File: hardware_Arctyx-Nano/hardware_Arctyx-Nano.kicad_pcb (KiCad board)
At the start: 4 copper layers, 21 x 51 mm, 74 parts, among them J1 USB_C_Receptacle_USB2.0_16P, J2 Conn_01x20_Pin, J3 Conn_01x20_Pin, SW1 SW_Push, U1 ICE40UP5K-SG48ITR, U2 RP2350A-QFN60, U3 W25Q128JVP, U4 RT8075ZQW, U5 TJ-S1608SW6TDSLCCYRGB-A5, Y1 Crystal_GND24

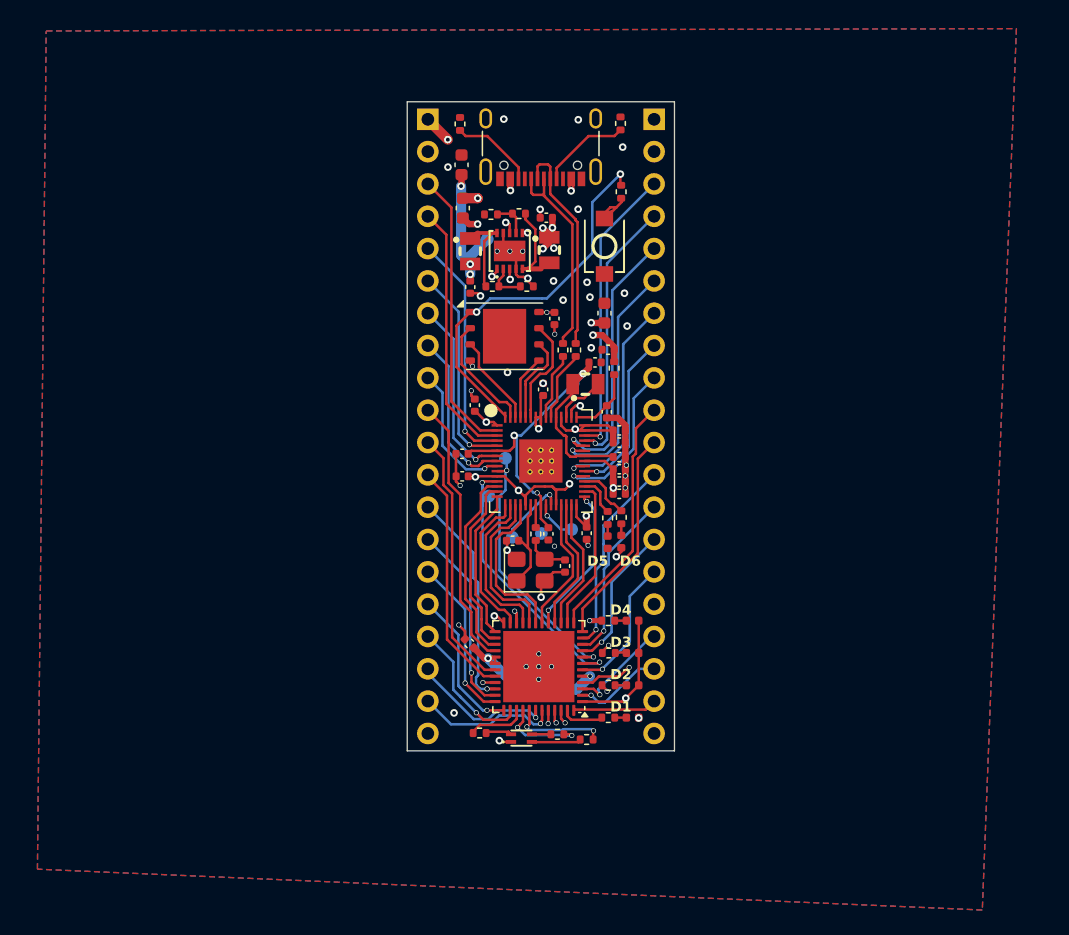
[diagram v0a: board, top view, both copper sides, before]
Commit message: production files generation and branding
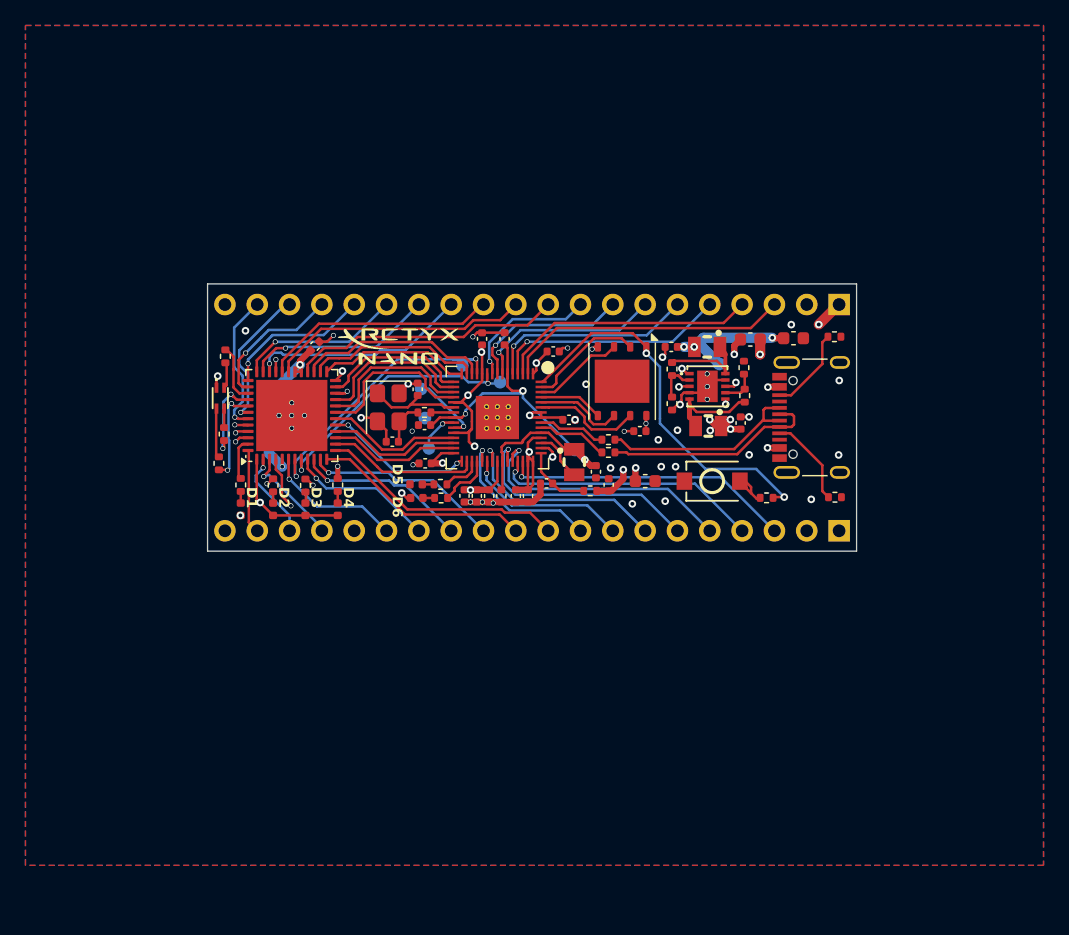
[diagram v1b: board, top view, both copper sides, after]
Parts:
- added G***: LOGO, LOGO, F.Cu at (149.3, 70.2)
- R11: value 51k -> 100k
- R12: value R -> 22k
- moved R15 36.1 mm to (135.2, 78.4), turned to -90 degrees
- moved R13 35.7 mm to (135.7, 70.0), turned to 90 degrees
- moved U5 35.7 mm to (135.3, 73.3), turned to -90 degrees
- moved J3 35.5 mm to (183.9, 83.7), turned to 90 degrees
- moved J2 35.4 mm to (183.9, 65.9), turned to 90 degrees
- moved R14 35.2 mm to (135.6, 76.1), turned to -90 degrees
- moved D1 34.9 mm to (136.9, 82.0), turned to -90 degrees
- moved R16 34.2 mm to (136.9, 80.1), turned to -90 degrees
- moved R1 33.9 mm to (183.6, 81.1), turned to 0 degrees
- moved R2 33.8 mm to (183.6, 68.5), turned to 0 degrees
- moved J1 31.7 mm to (182.9, 74.8), turned to 90 degrees
- moved D2 31.5 mm to (139.5, 82.0), turned to -90 degrees
- moved R17 30.7 mm to (139.5, 80.1), turned to -90 degrees
- moved C24 29.4 mm to (180.4, 68.6), turned to 0 degrees
- moved D3 28.1 mm to (142.0, 82.0), turned to -90 degrees
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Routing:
- net GND: track 28.7 -> 31.8 mm
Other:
- board size 21 x 51 mm -> 51 x 21 mm
- board text added: "Keyaan Was Here"
